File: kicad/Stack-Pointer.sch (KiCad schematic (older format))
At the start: 38 parts, among them U137 74LS245, U138 74LS173, U139 74LS173, U140 74LS245, U141 74LS173, U142 74LS173

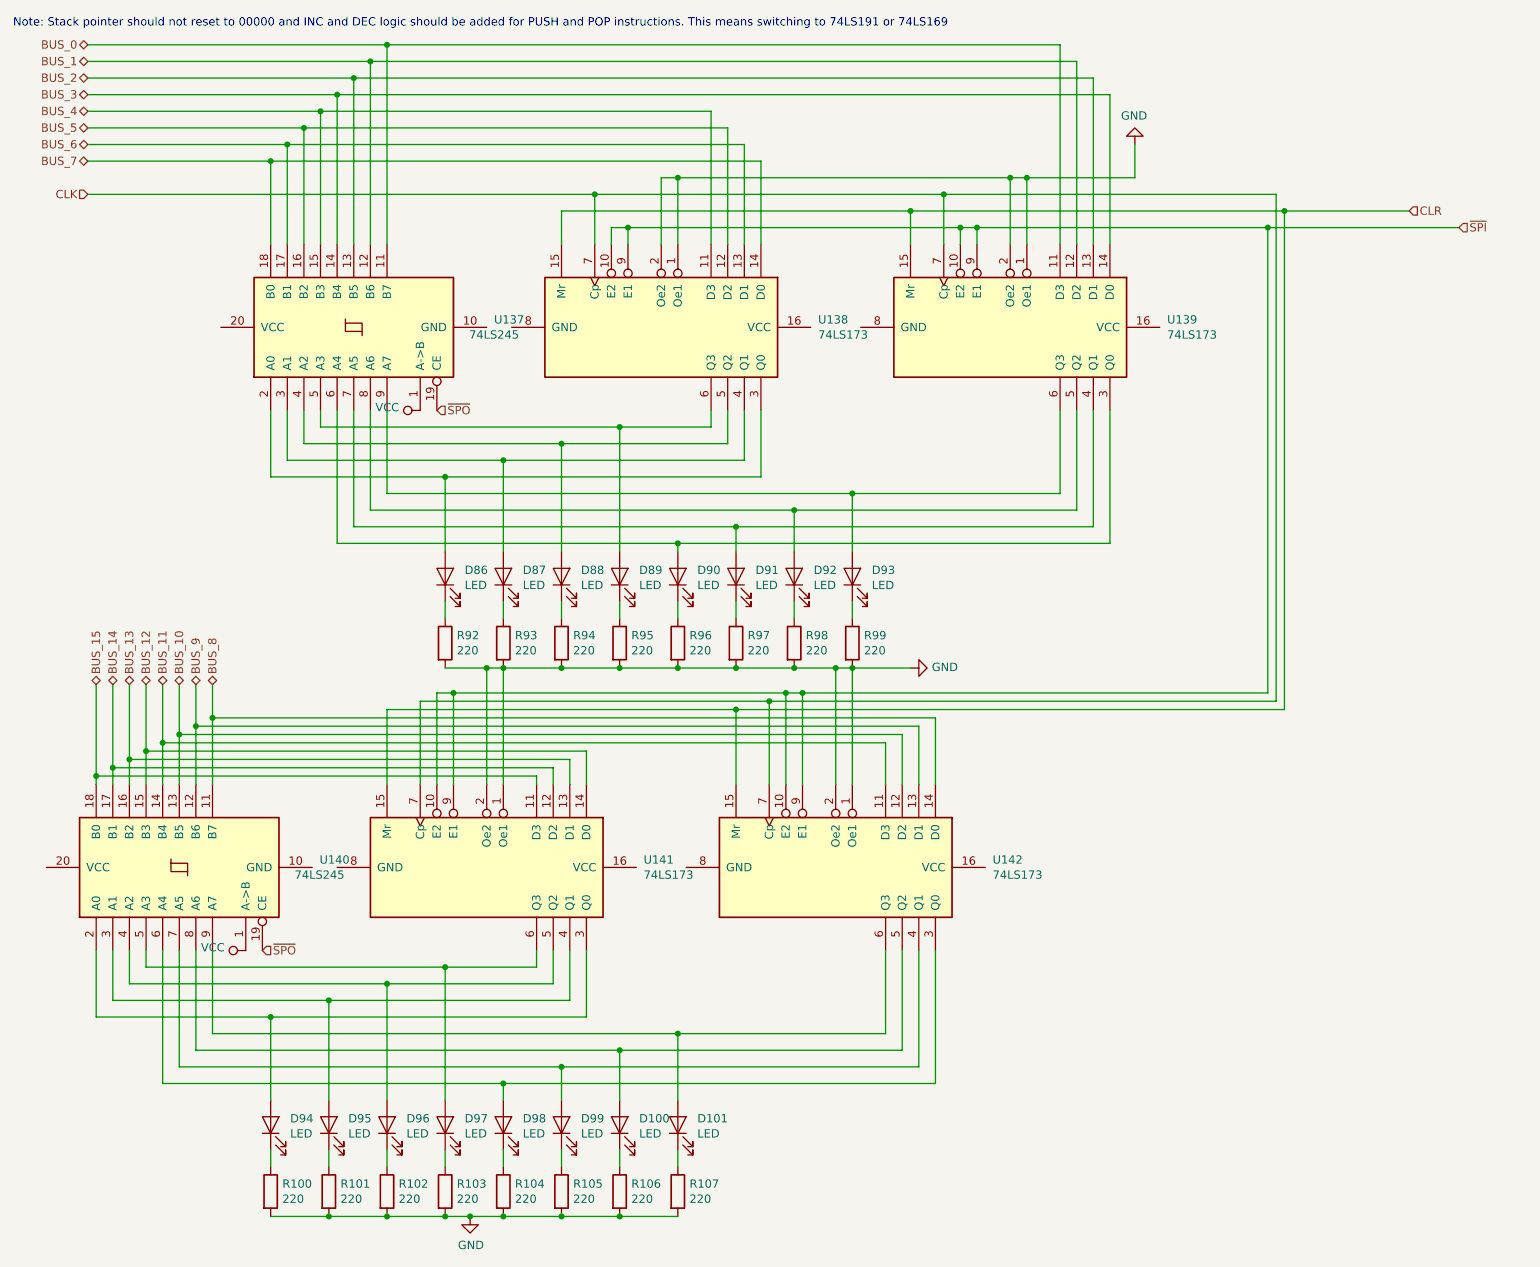
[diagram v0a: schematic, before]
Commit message: Finish todo list
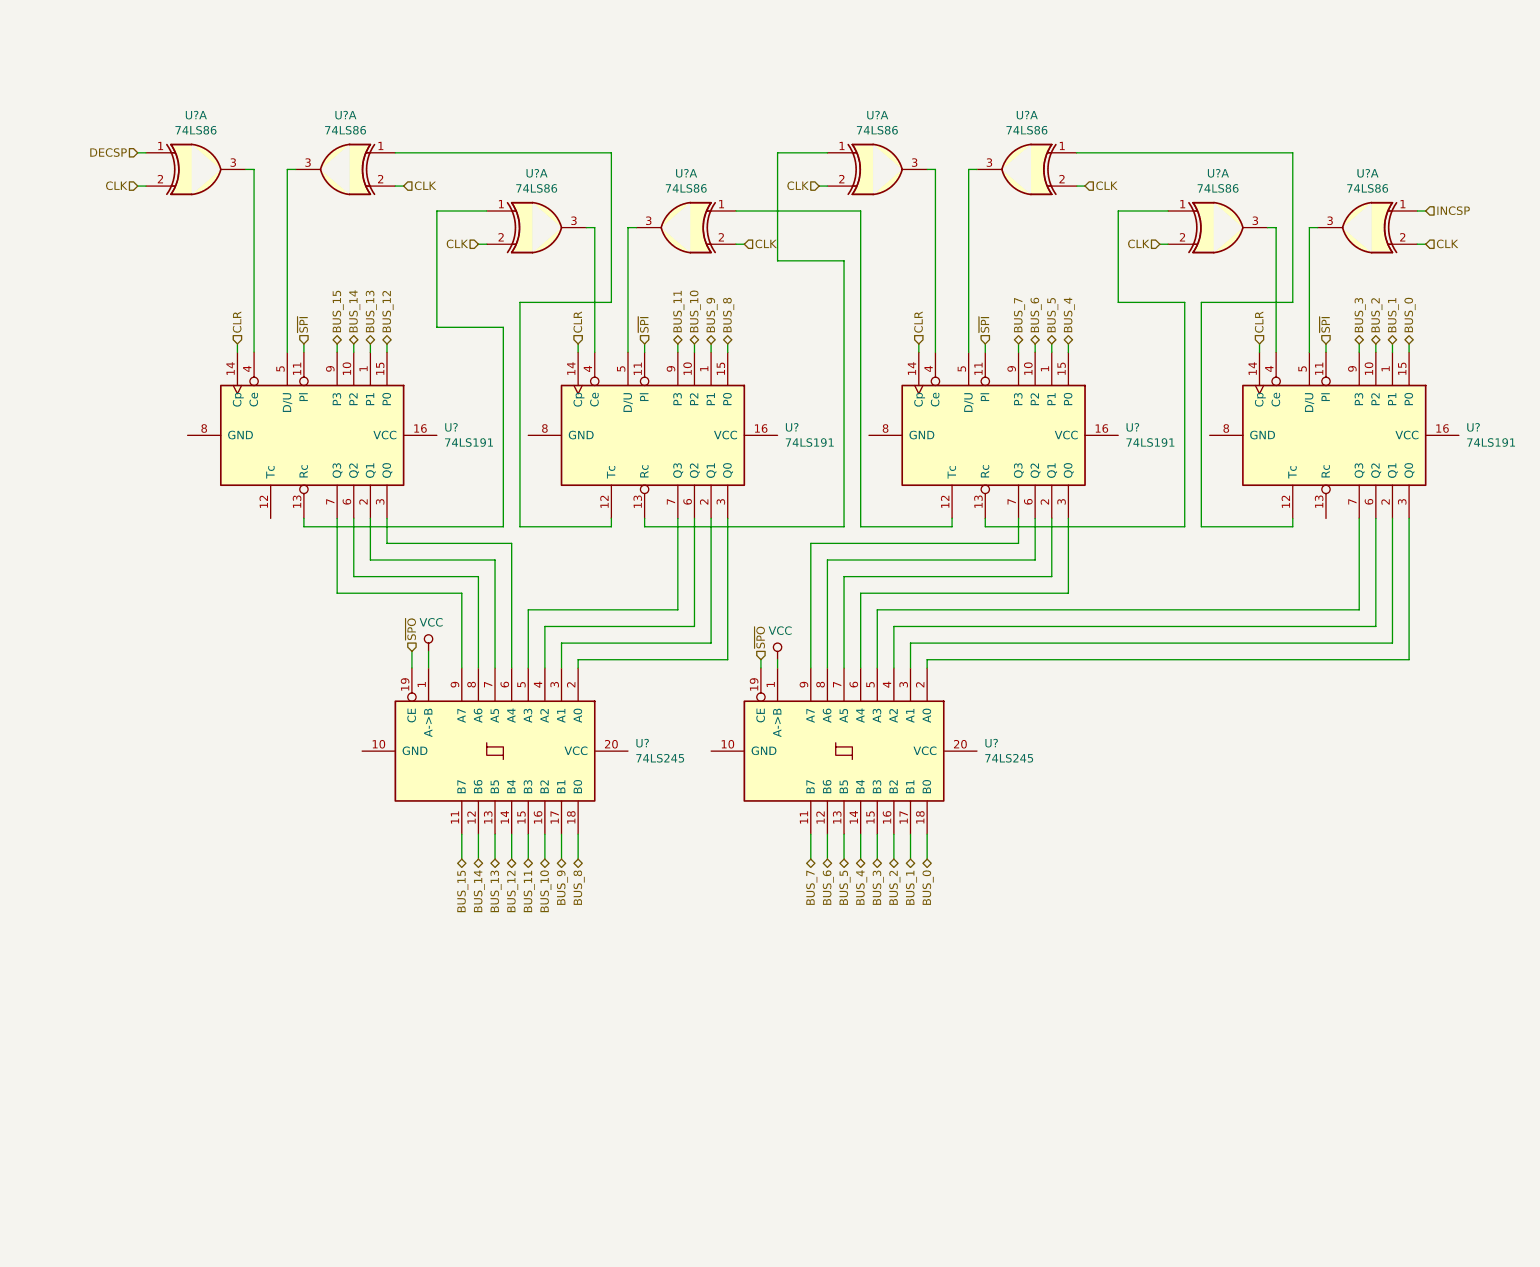
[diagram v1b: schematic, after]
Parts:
- removed D100, D101, D86, D87, D88, D89, D90, D91, D92, D93, D94, D95, D96, D97, D98, D99: LED, symbol Device:LED
- removed R100, R101, R102, R103, R104, R105, R106, R107, R92, R93, R94, R95, R96, R97, R98, R99: 220, symbol Device:R
- removed U137, U140: 74LS245, symbol 74xx:74LS245
- removed U138, U139, U141, U142: 74LS173, symbol 74xx:74LS173
- added U? (x2): 74LS245, symbol 74xx:74LS245
- added U? (x4): 74LS191, symbol 74xx:74LS191
- added U? (x8): 74LS86, symbol 74xx:74LS86
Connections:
- net BUS_0: now also U?.15 (P0), U?.18 (B0)
- net BUS_1: now also U?.1 (P1), U?.17 (B1)
- net BUS_10: now also U?.10 (P2), U?.16 (B2)
- net BUS_11: now also U?.15 (B3), U?.9 (P3)
- net BUS_12: now also U?.14 (B4), U?.15 (P0)
- net BUS_13: now also U?.1 (P1), U?.13 (B5)
- net BUS_14: now also U?.10 (P2), U?.12 (B6)
- net BUS_15: now also U?.11 (B7), U?.9 (P3)
- net BUS_2: now also U?.10 (P2), U?.16 (B2)
- net BUS_3: now also U?.15 (B3), U?.9 (P3)
- net BUS_4: now also U?.14 (B4), U?.15 (P0)
- net BUS_5: now also U?.1 (P1), U?.13 (B5)
- net BUS_6: now also U?.10 (P2), U?.12 (B6)
- net BUS_7: now also U?.11 (B7), U?.9 (P3)
- net BUS_8: now also U?.15 (P0), U?.18 (B0)
- net BUS_9: now also U?.1 (P1), U?.17 (B1)
- net CLK: now also U?.2, U?.2, U?.2, U?.2, U?.2, U?.2, U?.2, U?.2
- net CLR: now also U?.14 (Cp), U?.14 (Cp), U?.14 (Cp), U?.14 (Cp)
- net VCC: now also U?.1 (A->B), U?.1 (A->B)
- net ~SPI~: now also U?.11 (Pl), U?.11 (Pl), U?.11 (Pl), U?.11 (Pl)
- net ~SPO~: now also U?.19 (CE), U?.19 (CE)
- new net: U?.2 (A0), U?.3 (Q0) (x2)
- new net: U?.2 (Q1), U?.3 (A1) (x2)
- new net: U?.4 (A2), U?.6 (Q2) (x2)
- new net: U?.5 (A3), U?.7 (Q3) (x2)
- new net: U?.3 (Q0), U?.6 (A4) (x2)
- new net: U?.2 (Q1), U?.7 (A5) (x2)
- new net: U?.6 (Q2), U?.8 (A6) (x2)
- new net: U?.7 (Q3), U?.9 (A7) (x2)
- new net: U?.1, U?.12 (Tc) (x3)
- new net: U?.3, U?.4 (Ce) (x4)
- new net: U?.3, U?.5 (D/U) (x4)
- new net: U?.1, U?.13 (Rc) (x3)
- new net DECSP: U?.1
- new net INCSP: U?.1
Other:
- note removed: "Note: Stack pointer should not reset to 00000 and INC and DEC logic should be added for PUSH and POP instructions. This means switching to 74LS191 or 74LS169"
